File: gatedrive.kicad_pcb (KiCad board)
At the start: 2 copper layers, 200.7 x 101.6 mm, 154 parts, among them IC1 uA741_RevA_14Sep2012, IC10 IXDD614PI, IC11 HCPL-316J, IC12 IXDD614PI, IC13 HCPL-316J, IC14 IXDD614PI, IC15 HCPL-316J, IC16 IXDD614PI, IC3 HCPL-316J, IC4 IXDD614PI, IC5 HCPL-316J, IC6 IXDD614PI, IC7 HCPL-316J, IC8 IXDD614PI, IC9 HCPL-316J, P1 Mic General Connector, P10 CONN_01X03, P11 CONN_01X03, P12 CONN_01X03, P13 CONN_01X03, P14 CONN_01X03, P15 CONN_01X03, P16 CONN_01X03, P17 CONN_01X03, P18 FromShuntResistor, P2 FromNtc, P4 CONN_01X03, P5 CONN_01X03, P6 CONN_01X03, P7 CONN_01X03, P8 CONN_01X03, P9 CONN_01X03, U2 LM393

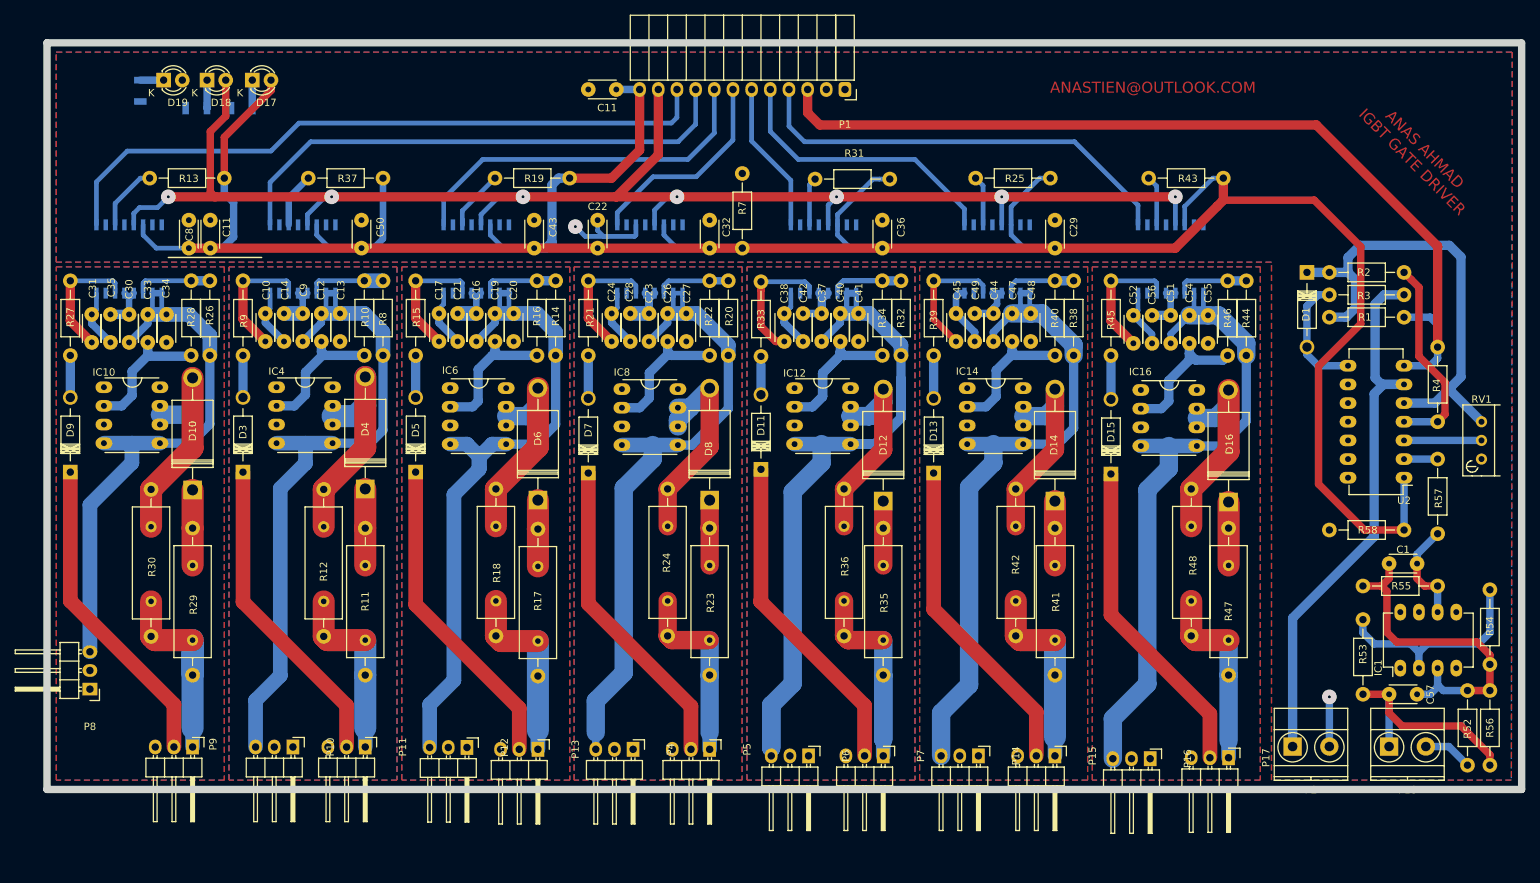
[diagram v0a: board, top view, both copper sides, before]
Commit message: yet another enhancements .
the protection section still is incomplete.
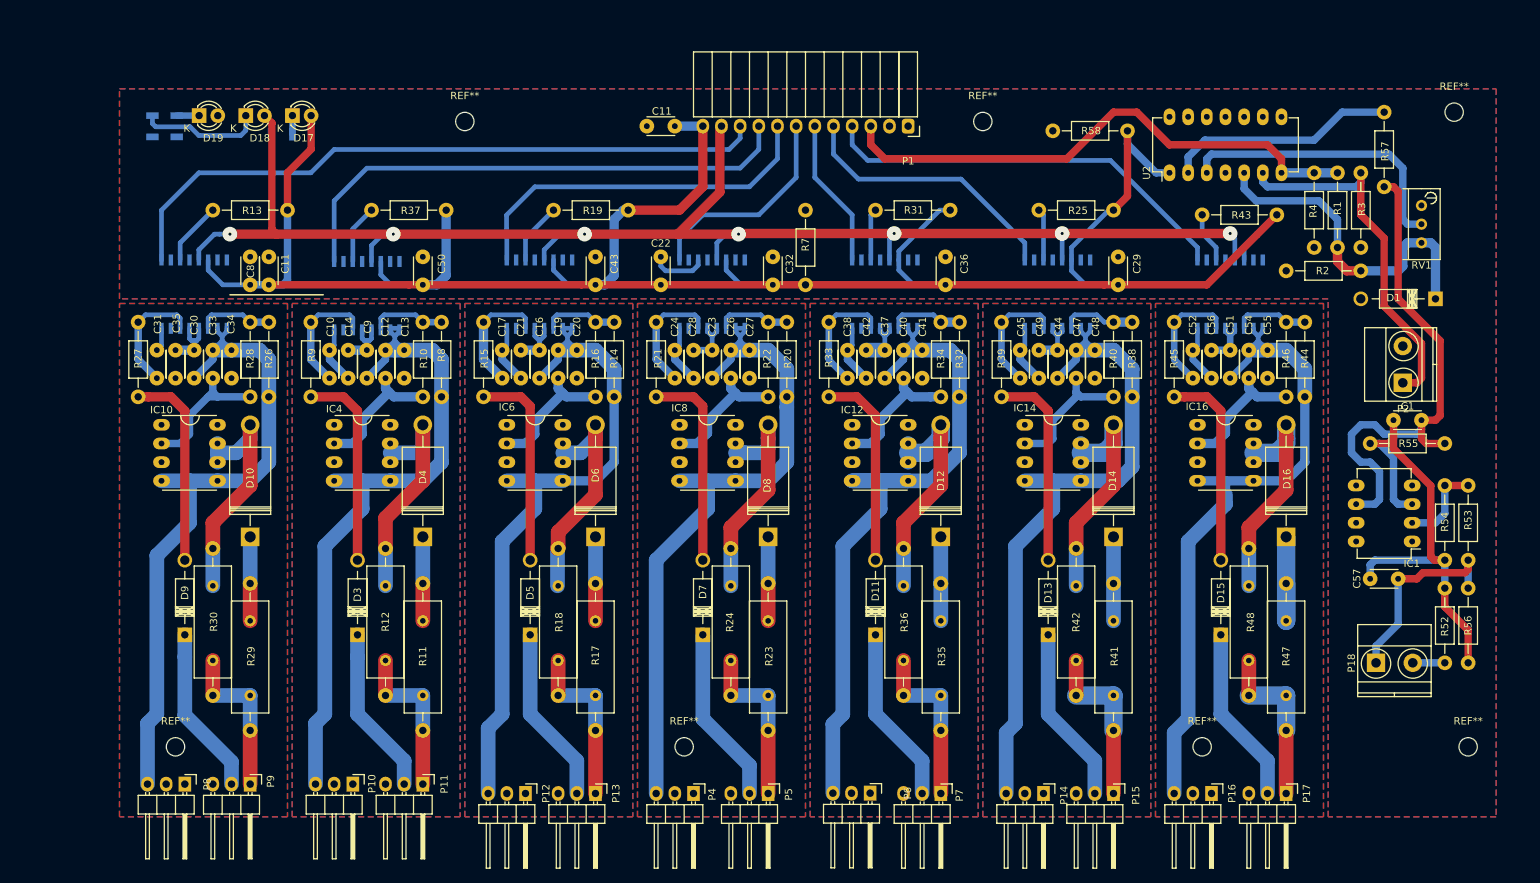
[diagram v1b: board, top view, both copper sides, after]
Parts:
- added REF**: MountingHole_2.5mm, Mounting_Holes:MountingHole_2.5mm, F.Cu at (125.7, 134.0)
- added REF**: MountingHole_2.5mm, Mounting_Holes:MountingHole_2.5mm, F.Cu at (196.2, 134.0)
- added REF**: MountingHole_2.5mm, Mounting_Holes:MountingHole_2.5mm, F.Cu at (230.5, 47.6)
- added REF**: MountingHole_2.5mm, Mounting_Holes:MountingHole_2.5mm, F.Cu at (166.4, 48.9)
- added REF**: MountingHole_2.5mm, Mounting_Holes:MountingHole_2.5mm, F.Cu at (95.9, 48.9)
- added REF**: MountingHole_2.5mm, Mounting_Holes:MountingHole_2.5mm, F.Cu at (232.4, 134.0)
- added REF**: MountingHole_2.5mm, Mounting_Holes:MountingHole_2.5mm, F.Cu at (56.5, 134.0)
- moved R58 66.1 mm to (175.9, 50.2)
- moved U2 52.3 mm to (191.8, 55.9), turned to 90 degrees
- moved P2 51.7 mm to (223.5, 84.5), turned to 90 degrees
- moved R57 47.8 mm to (221.0, 57.8)
- moved RV1 35.5 mm to (226.1, 60.3), turned to 180 degrees
- moved R4 29.1 mm to (211.5, 66.0)
- moved D11 27.4 mm to (151.8, 118.7)
- moved D3 27.1 mm to (81.3, 118.7)
- moved D5 27.1 mm to (104.8, 118.7)
- moved D9 27.1 mm to (57.8, 118.7)
- moved D13 27.0 mm to (175.3, 118.7)
- moved D7 27.0 mm to (128.3, 118.7)
- moved D15 26.5 mm to (198.8, 118.7)
- moved R53 23.2 mm to (232.4, 108.6)
- moved C1 19.5 mm to (226.1, 89.5)
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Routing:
- net ~FAULT: track 380.7 -> 317.9 mm
- net Net-(C1-Pad1): track 14.0 -> 70.6 mm
- net ~OVERTEMP: track 124.7 -> 74.0 mm
- net MICSUPP: track 93.1 -> 53.7 mm, vias 2 -> 0
- net Net-(RV1-Pad2): track 10.5 -> 39.4 mm
- net Net-(R57-Pad2): track 4.57 -> 31.4 mm
- net Net-(P2-Pad1): track 75.7 -> 50.6 mm
- net Net-(D11-Pad2): track 4.06 -> 27.1 mm
- net -5V4: track 123.9 -> 101.6 mm
- net Net-(D5-Pad2): track 5.71 -> 27.8 mm
- net Net-(D7-Pad2): track 5.84 -> 27.8 mm
- net Net-(D3-Pad2): track 5.71 -> 27.5 mm
- net Net-(D9-Pad2): track 5.71 -> 27.5 mm
- net Net-(D13-Pad2): track 5.84 -> 27.5 mm
- net Net-(D15-Pad2): track 5.97 -> 27.5 mm
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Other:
- board outline removed
- board text removed: "ANAS AHMAD IGBT GATE DRIVER"
- board text removed: "ANASTIEN@OUTLOOK.COM"

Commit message: packup
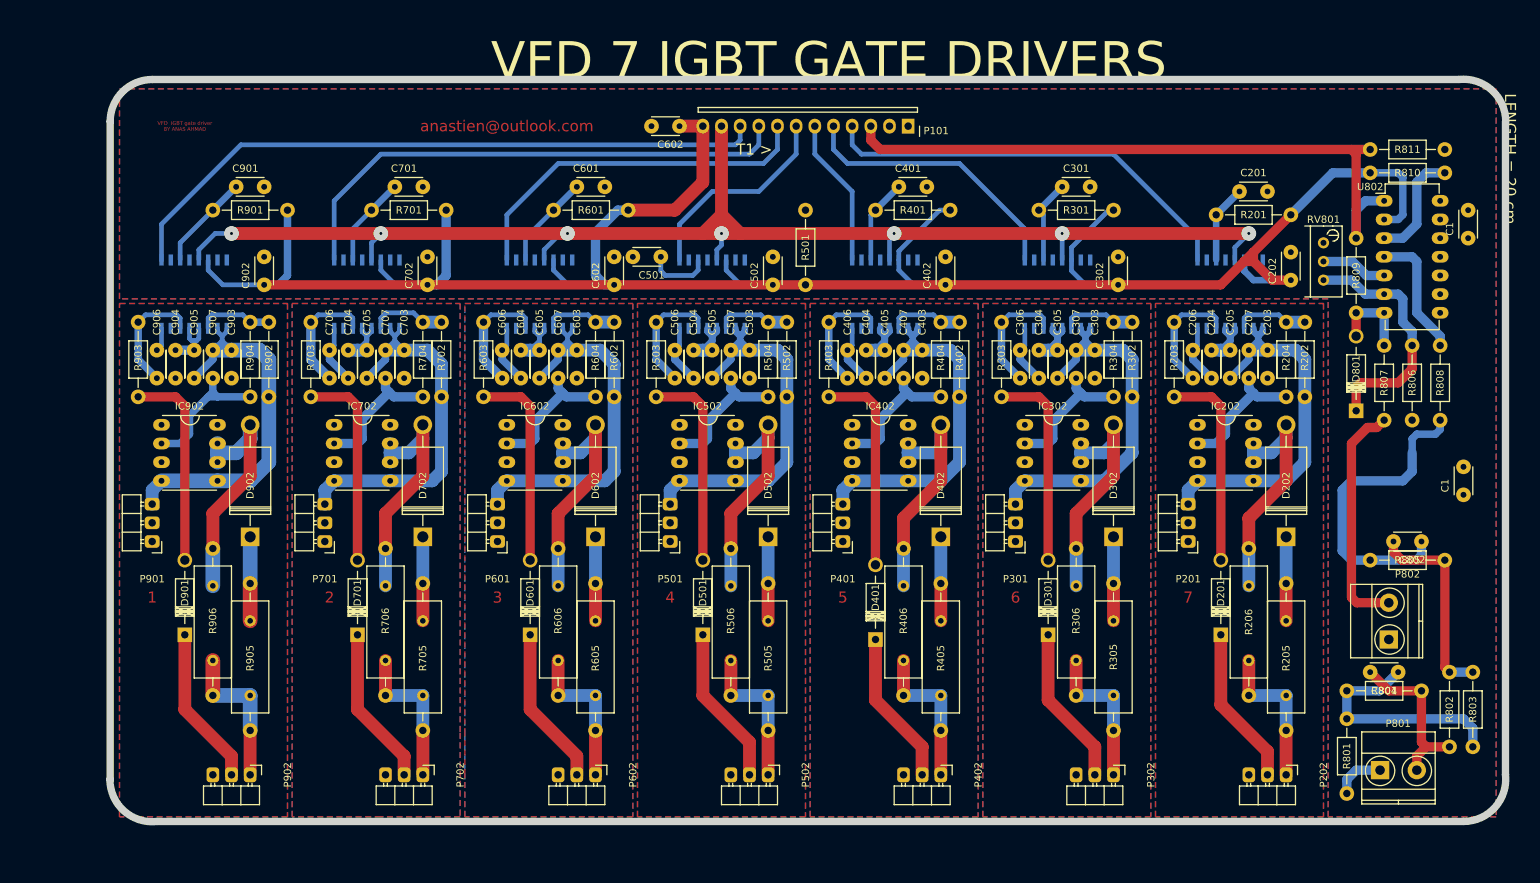
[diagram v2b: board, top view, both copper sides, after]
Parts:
- removed the C1 at (226.1, 89.5)
- removed C10, C17, C24, C31, C38, C45, C52: 100pF, gatedrive:C_Disc
- removed C11 (x2), C32: 330pF, gatedrive:C_Disc
- removed C12, C19, C26, C33, C40, C47, C54: 10nF, gatedrive:C_Disc
- removed C13, C14, C16, C20, C21, C22, C23, C27, C28, C29, C30, C34, C35, C36, C37, C41, C42, C43, C44, C48, C49, C50, C51, C55, C56, C8, C9: 0.1uF, gatedrive:C_Disc
- removed C57: 330p, gatedrive:C_Disc
- removed D1: ZENER, Diodes_ThroughHole:Diode_DO-41_SOD81_Horizontal_RM10
- removed D10, D12, D14, D16, D4, D6, D8: ~, Diodes_ThroughHole:Diode_DO-201AD_Horizontal_RM15
- removed D11, D13, D15, D3, D5, D7, D9: RGPO2-20, Diodes_ThroughHole:Diode_DO-41_SOD81_Horizontal_RM10
- removed D17, D18, D19: LED, LEDs:LED-3MM
- removed IC1: uA741_RevA_14Sep2012, Housings_DIP:DIP-8_W7.62mm_LongPads
- removed IC10, IC12, IC14, IC16, IC4, IC6, IC8: IXDD614PI, gatedrive:DIP-8_W7.62mm_LongPads
- removed IC11, IC13, IC15, IC3, IC5, IC7, IC9: HCPL-316J, Housings_SOIC:SOIC-16_7.5x10.3mm_Pitch1.27mm
- removed P1: Mic General Connector, Socket_Strips:Socket_Strip_Angled_1x12
- removed P10, P11, P12, P13, P14, P15, P16, P17, P4, P5, P6, P7, P8, P9: CONN_01X03, Pin_Headers:Pin_Header_Angled_1x03
- removed P18: FromShuntResistor, Terminal_Blocks:TerminalBlock_Pheonix_MKDS1.5-2pol
- removed P2: FromNtc, Terminal_Blocks:TerminalBlock_Pheonix_MKDS1.5-2pol
- removed R1: 2.2MEG, Resistors_ThroughHole:Resistor_Horizontal_RM10mm
- removed R10, R15, R16, R21, R22, R27, R28, R33, R34, R39, R40, R45, R46, R9: 100, Resistors_ThroughHole:Resistor_Horizontal_RM10mm
- removed R11, R17, R23, R29, R35, R41, R47: 60, gatedrive:Resistor_multi
- removed R12, R18, R24, R30, R36, R42, R48: 30ohm ,0.5W, gatedrive:Resistor_multi
- removed R13, R19, R25, R3, R31, R37, R43, R7: 10K, Resistors_ThroughHole:Resistor_Horizontal_RM10mm
- removed R14, R20, R26, R32, R38, R44, R8: 25K, Resistors_ThroughHole:Resistor_Horizontal_RM10mm
- removed R2: 560, Resistors_ThroughHole:Resistor_Horizontal_RM10mm
- removed R4, R52, R53, R55, R56, R57, R58: 1.24k, Resistors_ThroughHole:Resistor_Horizontal_RM10mm
- removed R49, R50, R51: R, Resistors_SMD:R_1206
- removed R54: 20k, Resistors_ThroughHole:Resistor_Horizontal_RM10mm
- removed REF** (x7): MountingHole_2.5mm, Mounting_Holes:MountingHole_2.5mm
- removed RV1: POT, Potentiometers:Potentiometer_Bourns_3296W_3-8Zoll_Inline_ScrewUp
- removed U2: LM393, Housings_DIP:DIP-14_W7.62mm_LongPads
- added C1: 0.1u, gatedrive:C_Disc, F.Cu at (231.8, 99.7)
- added C1: 0.1u, gatedrive:C_Disc, F.Cu at (232.4, 64.8)
- added C201: 0.1uF, gatedrive:C_Disc, F.Cu at (201.3, 58.4)
- added C202: 330pF, gatedrive:C_Disc, F.Cu at (208.3, 70.5)
- added C203: 0.1uF, gatedrive:C_Disc, F.Cu at (205.1, 80.0)
- added C204: 0.1uF, gatedrive:C_Disc, F.Cu at (197.5, 83.8)
- added C205: 0.1uF, gatedrive:C_Disc, F.Cu at (200.0, 80.0)
- added C206: 100pF, gatedrive:C_Disc, F.Cu at (194.9, 83.8)
- added C207: 10nF, gatedrive:C_Disc, F.Cu at (202.6, 83.8)
- added C301: 0.1uF, gatedrive:C_Disc, F.Cu at (177.2, 57.8)
- added C302: 330pF, gatedrive:C_Disc, F.Cu at (184.8, 71.1)
- added C303: 0.1uF, gatedrive:C_Disc, F.Cu at (181.6, 80.0)
- added C304: 0.1uF, gatedrive:C_Disc, F.Cu at (174.0, 83.8)
- added C305: 0.1uF, gatedrive:C_Disc, F.Cu at (176.5, 80.0)
- added C306: 100pF, gatedrive:C_Disc, F.Cu at (171.4, 83.8)
- added C307: 10nF, gatedrive:C_Disc, F.Cu at (179.1, 83.8)
- added C401: 0.1uF, gatedrive:C_Disc, F.Cu at (154.9, 57.8)
- added C402: 330pF, gatedrive:C_Disc, F.Cu at (161.3, 71.1)
- added C403: 0.1uF, gatedrive:C_Disc, F.Cu at (158.1, 80.0)
- added C404: 0.1uF, gatedrive:C_Disc, F.Cu at (150.5, 83.8)
- added C405: 0.1uF, gatedrive:C_Disc, F.Cu at (153.0, 80.0)
- added C406: 100pF, gatedrive:C_Disc, F.Cu at (148.0, 83.8)
- added C407: 10nF, gatedrive:C_Disc, F.Cu at (155.6, 83.8)
- added C501: 0.1uF, gatedrive:C_Disc, F.Cu at (122.6, 67.3)
- added C502: 330pF, gatedrive:C_Disc, F.Cu at (137.8, 71.1)
- added C503: 0.1uF, gatedrive:C_Disc, F.Cu at (134.6, 80.0)
- added C504: 0.1uF, gatedrive:C_Disc, F.Cu at (127.0, 83.8)
- added C505: 0.1uF, gatedrive:C_Disc, F.Cu at (129.5, 80.0)
- added C506: 100pF, gatedrive:C_Disc, F.Cu at (124.5, 83.8)
- added C507: 10nF, gatedrive:C_Disc, F.Cu at (132.1, 83.8)
- added C601: 0.1uF, gatedrive:C_Disc, F.Cu at (111.1, 57.8)
- added C602: 330pF, gatedrive:C_Disc, F.Cu at (125.1, 49.5)
- added C602: 330pF, gatedrive:C_Disc, F.Cu at (116.2, 71.1)
- added C603: 0.1uF, gatedrive:C_Disc, F.Cu at (111.1, 80.0)
- added C604: 0.1uF, gatedrive:C_Disc, F.Cu at (103.5, 83.8)
- added C605: 0.1uF, gatedrive:C_Disc, F.Cu at (106.0, 80.0)
- added C606: 100pF, gatedrive:C_Disc, F.Cu at (101.0, 83.8)
- added C607: 10nF, gatedrive:C_Disc, F.Cu at (108.6, 83.8)
- added C701: 0.1uF, gatedrive:C_Disc, F.Cu at (86.4, 57.8)
- added C702: 330pF, gatedrive:C_Disc, F.Cu at (90.8, 71.1)
- added C703: 0.1uF, gatedrive:C_Disc, F.Cu at (87.6, 80.0)
- added C704: 0.1uF, gatedrive:C_Disc, F.Cu at (80.0, 83.8)
- added C705: 0.1uF, gatedrive:C_Disc, F.Cu at (82.5, 80.0)
- added C706: 100pF, gatedrive:C_Disc, F.Cu at (77.5, 83.8)
- added C707: 10nF, gatedrive:C_Disc, F.Cu at (85.1, 83.8)
- added C801: 33pf, gatedrive:C_Disc, F.Cu at (219.1, 123.8)
- added C802: 33p, gatedrive:C_Disc, F.Cu at (226.1, 106.0)
- added C901: 0.1uF, gatedrive:C_Disc, F.Cu at (64.8, 57.8)
- added C902: 330pF, gatedrive:C_Disc, F.Cu at (68.6, 71.1)
- added C903: 0.1uF, gatedrive:C_Disc, F.Cu at (64.1, 80.0)
- added C904: 0.1uF, gatedrive:C_Disc, F.Cu at (56.5, 83.8)
- added C905: 0.1uF, gatedrive:C_Disc, F.Cu at (59.1, 80.0)
- added C906: 100pF, gatedrive:C_Disc, F.Cu at (54.0, 83.8)
- added C907: 10nF, gatedrive:C_Disc, F.Cu at (61.6, 83.8)
- added D201: RGPO2-20, Diodes_ThroughHole:Diode_DO-41_SOD81_Horizontal_RM10, F.Cu at (198.8, 118.7)
- added D202: ~, Diodes_ThroughHole:Diode_DO-201AD_Horizontal_RM15, F.Cu at (207.6, 105.4)
- added D301: RGPO2-20, Diodes_ThroughHole:Diode_DO-41_SOD81_Horizontal_RM10, F.Cu at (175.3, 118.7)
- added D302: ~, Diodes_ThroughHole:Diode_DO-201AD_Horizontal_RM15, F.Cu at (184.2, 105.4)
- added D401: RGPO2-20, Diodes_ThroughHole:Diode_DO-41_SOD81_Horizontal_RM10, F.Cu at (151.8, 119.4)
- added D402: ~, Diodes_ThroughHole:Diode_DO-201AD_Horizontal_RM15, F.Cu at (160.7, 105.4)
- added D501: RGPO2-20, Diodes_ThroughHole:Diode_DO-41_SOD81_Horizontal_RM10, F.Cu at (128.3, 118.7)
- added D502: ~, Diodes_ThroughHole:Diode_DO-201AD_Horizontal_RM15, F.Cu at (137.2, 105.4)
- added D601: RGPO2-20, Diodes_ThroughHole:Diode_DO-41_SOD81_Horizontal_RM10, F.Cu at (104.8, 118.7)
- added D602: ~, Diodes_ThroughHole:Diode_DO-201AD_Horizontal_RM15, F.Cu at (113.7, 105.4)
- added D701: RGPO2-20, Diodes_ThroughHole:Diode_DO-41_SOD81_Horizontal_RM10, F.Cu at (81.3, 118.7)
- added D702: ~, Diodes_ThroughHole:Diode_DO-201AD_Horizontal_RM15, F.Cu at (90.2, 105.4)
- added D801: ZENER, Diodes_ThroughHole:Diode_DO-41_SOD81_Horizontal_RM10, F.Cu at (217.2, 88.3)
- added D901: RGPO2-20, Diodes_ThroughHole:Diode_DO-41_SOD81_Horizontal_RM10, F.Cu at (57.8, 118.7)
- added D902: ~, Diodes_ThroughHole:Diode_DO-201AD_Horizontal_RM15, F.Cu at (66.7, 105.4)
- added IC201: HCPL-316J, Housings_SOIC:SOIC-16_7.5x10.3mm_Pitch1.27mm, B.Cu at (200.0, 72.4)
- added IC202: IXDD614PI, gatedrive:DIP-8_W7.62mm_LongPads, F.Cu at (195.6, 90.2)
- added IC301: HCPL-316J, Housings_SOIC:SOIC-16_7.5x10.3mm_Pitch1.27mm, B.Cu at (176.5, 72.4)
- added IC302: IXDD614PI, gatedrive:DIP-8_W7.62mm_LongPads, F.Cu at (172.1, 90.2)
- added IC401: HCPL-316J, Housings_SOIC:SOIC-16_7.5x10.3mm_Pitch1.27mm, B.Cu at (153.0, 72.4)
- added IC402: IXDD614PI, gatedrive:DIP-8_W7.62mm_LongPads, F.Cu at (148.6, 90.2)
- added IC501: HCPL-316J, Housings_SOIC:SOIC-16_7.5x10.3mm_Pitch1.27mm, B.Cu at (129.5, 72.4)
- added IC502: IXDD614PI, gatedrive:DIP-8_W7.62mm_LongPads, F.Cu at (125.1, 90.2)
- added IC601: HCPL-316J, Housings_SOIC:SOIC-16_7.5x10.3mm_Pitch1.27mm, B.Cu at (106.0, 72.4)
- added IC602: IXDD614PI, gatedrive:DIP-8_W7.62mm_LongPads, F.Cu at (101.6, 90.2)
- added IC701: HCPL-316J, Housings_SOIC:SOIC-16_7.5x10.3mm_Pitch1.27mm, B.Cu at (82.5, 72.4)
- added IC702: IXDD614PI, gatedrive:DIP-8_W7.62mm_LongPads, F.Cu at (78.1, 90.2)
- added IC901: HCPL-316J, Housings_SOIC:SOIC-16_7.5x10.3mm_Pitch1.27mm, B.Cu at (59.1, 72.4)
- added IC902: IXDD614PI, gatedrive:DIP-8_W7.62mm_LongPads, F.Cu at (54.6, 90.2)
- added P101: Mic General Connector, Socket_Strips:Socket_Strip_Angled_1x12, F.Cu at (156.2, 49.5)
- added P201: CONN_01X03, gatedrive:conn, F.Cu at (194.3, 106.0)
- added P202: CONN_01X03, gatedrive:conn, F.Cu at (207.6, 137.8)
- added P301: CONN_01X03, gatedrive:conn, F.Cu at (170.8, 106.0)
- added P302: CONN_01X03, gatedrive:conn, F.Cu at (184.2, 137.8)
- added P401: CONN_01X03, gatedrive:conn, F.Cu at (147.3, 106.0)
- added P402: CONN_01X03, gatedrive:conn, F.Cu at (160.7, 137.8)
- added P501: CONN_01X03, gatedrive:conn, F.Cu at (123.8, 106.0)
- added P502: CONN_01X03, gatedrive:conn, F.Cu at (137.2, 137.8)
- added P601: CONN_01X03, gatedrive:conn, F.Cu at (100.3, 106.0)
- added P602: CONN_01X03, gatedrive:conn, F.Cu at (113.7, 137.8)
- added P701: CONN_01X03, gatedrive:conn, F.Cu at (76.8, 106.0)
- added P702: CONN_01X03, gatedrive:conn, F.Cu at (90.2, 137.8)
- added P801: FromShuntResistor, Terminal_Blocks:TerminalBlock_Pheonix_MKDS1.5-2pol, F.Cu at (220.4, 137.2)
- added P802: FromNtc, Terminal_Blocks:TerminalBlock_Pheonix_MKDS1.5-2pol, F.Cu at (221.6, 119.4)
- added P901: CONN_01X03, gatedrive:conn, F.Cu at (53.3, 106.0)
- added P902: CONN_01X03, gatedrive:conn, F.Cu at (66.7, 137.8)
- added R201: 10K, Resistors_ThroughHole:Resistor_Horizontal_RM10mm, F.Cu at (208.3, 61.6)
- added R202: 25K, Resistors_ThroughHole:Resistor_Horizontal_RM10mm, F.Cu at (210.2, 86.4)
- added R203: 100, Resistors_ThroughHole:Resistor_Horizontal_RM10mm, F.Cu at (192.4, 76.2)
- added R204: 100, Resistors_ThroughHole:Resistor_Horizontal_RM10mm, F.Cu at (207.6, 86.4)
- added R205: 60, gatedrive:Resistor_multi, F.Cu at (207.6, 111.8)
- added R206: 30ohm ,0.5W, gatedrive:Resistor_multi, F.Cu at (202.6, 107.0)
- added R301: 10K, Resistors_ThroughHole:Resistor_Horizontal_RM10mm, F.Cu at (184.2, 61.0)
- added R302: 25K, Resistors_ThroughHole:Resistor_Horizontal_RM10mm, F.Cu at (186.7, 86.4)
- added R303: 100, Resistors_ThroughHole:Resistor_Horizontal_RM10mm, F.Cu at (168.9, 76.2)
- added R304: 100, Resistors_ThroughHole:Resistor_Horizontal_RM10mm, F.Cu at (184.2, 86.4)
- added R305: 60, gatedrive:Resistor_multi, F.Cu at (184.2, 111.8)
- added R306: 30ohm ,0.5W, gatedrive:Resistor_multi, F.Cu at (179.1, 107.0)
- added R401: 10K, Resistors_ThroughHole:Resistor_Horizontal_RM10mm, F.Cu at (161.9, 61.0)
- added R402: 25K, Resistors_ThroughHole:Resistor_Horizontal_RM10mm, F.Cu at (163.2, 86.4)
- added R403: 100, Resistors_ThroughHole:Resistor_Horizontal_RM10mm, F.Cu at (145.4, 76.2)
- added R404: 100, Resistors_ThroughHole:Resistor_Horizontal_RM10mm, F.Cu at (160.7, 86.4)
- added R405: 60, gatedrive:Resistor_multi, F.Cu at (160.7, 111.8)
- added R406: 30ohm ,0.5W, gatedrive:Resistor_multi, F.Cu at (155.6, 107.0)
- added R501: 10K, Resistors_ThroughHole:Resistor_Horizontal_RM10mm, F.Cu at (142.2, 71.1)
- added R502: 25K, Resistors_ThroughHole:Resistor_Horizontal_RM10mm, F.Cu at (139.7, 86.4)
- added R503: 100, Resistors_ThroughHole:Resistor_Horizontal_RM10mm, F.Cu at (121.9, 76.2)
- added R504: 100, Resistors_ThroughHole:Resistor_Horizontal_RM10mm, F.Cu at (137.2, 86.4)
- added R505: 60, gatedrive:Resistor_multi, F.Cu at (137.2, 111.8)
- added R506: 30ohm ,0.5W, gatedrive:Resistor_multi, F.Cu at (132.1, 107.0)
- added R601: 10K, Resistors_ThroughHole:Resistor_Horizontal_RM10mm, F.Cu at (118.1, 61.0)
- added R602: 25K, Resistors_ThroughHole:Resistor_Horizontal_RM10mm, F.Cu at (116.2, 86.4)
- added R603: 100, Resistors_ThroughHole:Resistor_Horizontal_RM10mm, F.Cu at (98.4, 76.2)
- added R604: 100, Resistors_ThroughHole:Resistor_Horizontal_RM10mm, F.Cu at (113.7, 86.4)
- added R605: 60, gatedrive:Resistor_multi, F.Cu at (113.7, 111.8)
- added R606: 30ohm ,0.5W, gatedrive:Resistor_multi, F.Cu at (108.6, 107.0)
- added R701: 10K, Resistors_ThroughHole:Resistor_Horizontal_RM10mm, F.Cu at (93.3, 61.0)
- added R702: 25K, Resistors_ThroughHole:Resistor_Horizontal_RM10mm, F.Cu at (92.7, 86.4)
- added R703: 100, Resistors_ThroughHole:Resistor_Horizontal_RM10mm, F.Cu at (74.9, 76.2)
- added R704: 100, Resistors_ThroughHole:Resistor_Horizontal_RM10mm, F.Cu at (90.2, 86.4)
- added R705: 60, gatedrive:Resistor_multi, F.Cu at (90.2, 111.8)
- added R706: 30ohm ,0.5W, gatedrive:Resistor_multi, F.Cu at (85.1, 107.0)
- added R801: 1.24k, Resistors_ThroughHole:Resistor_Horizontal_RM10mm, F.Cu at (215.9, 140.3)
- added R802: 1.24k, Resistors_ThroughHole:Resistor_Horizontal_RM10mm, F.Cu at (229.9, 134.0)
- added R803: 20k, Resistors_ThroughHole:Resistor_Horizontal_RM10mm, F.Cu at (233.0, 134.0)
- added R804: 61.9k, Resistors_ThroughHole:Resistor_Horizontal_RM10mm, F.Cu at (226.1, 126.4)
- added R805: 61.9k, Resistors_ThroughHole:Resistor_Horizontal_RM10mm, F.Cu at (229.2, 108.6)
- added R806: 560, Resistors_ThroughHole:Resistor_Horizontal_RM10mm, F.Cu at (224.8, 89.5)
- added R807: 10K, Resistors_ThroughHole:Resistor_Horizontal_RM10mm, F.Cu at (221.0, 89.5)
- added R808: 10k, Resistors_ThroughHole:Resistor_Horizontal_RM10mm, F.Cu at (228.6, 89.5)
- added R809: 2.2MEG, Resistors_ThroughHole:Resistor_Horizontal_RM10mm, F.Cu at (217.2, 74.9)
- added R810: 10k, Resistors_ThroughHole:Resistor_Horizontal_RM10mm, F.Cu at (219.1, 55.9)
- added R811: 1.24k, Resistors_ThroughHole:Resistor_Horizontal_RM10mm, F.Cu at (229.2, 52.7)
- added R901: 10K, Resistors_ThroughHole:Resistor_Horizontal_RM10mm, F.Cu at (71.8, 61.0)
- added R902: 25K, Resistors_ThroughHole:Resistor_Horizontal_RM10mm, F.Cu at (69.2, 86.4)
- added R903: 100, Resistors_ThroughHole:Resistor_Horizontal_RM10mm, F.Cu at (51.4, 76.2)
- added R904: 100, Resistors_ThroughHole:Resistor_Horizontal_RM10mm, F.Cu at (66.7, 86.4)
- added R905: 60, gatedrive:Resistor_multi, F.Cu at (66.7, 111.8)
- added R906: 30ohm ,0.5W, gatedrive:Resistor_multi, F.Cu at (61.6, 107.0)
- added RV801: 10k, Potentiometers:Potentiometer_Bourns_3296W_3-8Zoll_Inline_ScrewUp, F.Cu at (212.7, 65.4)
- added U802: LM339, Housings_DIP:DIP-14_W7.62mm_LongPads, F.Cu at (221.0, 59.7)
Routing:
- net -5V5: track 106.9 -> 0.00 mm
- net -5V4: track 101.6 -> 0.00 mm
- net +5V: track 0.00 -> 96.4 mm
- net -5V7: track 95.6 -> 0.00 mm
- net -5V6: track 95.2 -> 0.00 mm
- net -5V3: track 94.3 -> 0.00 mm
- net -5V2: track 94.2 -> 0.00 mm
- net -5v8: track 93.2 -> 0.00 mm
- net /T8: track 91.2 -> 0.00 mm
- net /T1: track 0.00 -> 90.3 mm
- net Net-(C1-Pad1): track 70.6 -> 0.00 mm
- net Net-(C1-Pad2): track 66.9 -> 0.00 mm
- net MICSUPP: track 53.7 -> 0.00 mm
- net -5v3: track 0.00 -> 53.6 mm
- net -5v2: track 0.00 -> 53.6 mm
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- added copper zone on F.Cu, net +5V
- added copper zone on B.Cu, net 15V1
- added copper zone on F.Cu, net COM1
- added copper zone on B.Cu, net GND
- removed copper zone on B.Cu, net 15V8
- removed copper zone on F.Cu, net COM8
- removed copper zone on B.Cu, net GND1
- removed copper zone on F.Cu, net MICSUPP
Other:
- board outline added: 189.9 x 101 mm
- board text added: "1"
- board text added: "2"
- board text added: "3"
- board text added: "4"
- board text added: "5"
- board text added: "6"
- board text added: "7"
- board text added: "LENGTH = 20 cm"
- board text added: "T1 >"
- board text added: "VFD 7 IGBT GATE DRIVERS"
- board text added: "VFD IGBT gate driver BY ANAS AHMAD"
- board text added: "anastien@outlook.com"
